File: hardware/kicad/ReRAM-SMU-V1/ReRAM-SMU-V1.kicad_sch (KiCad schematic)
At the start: 0 parts

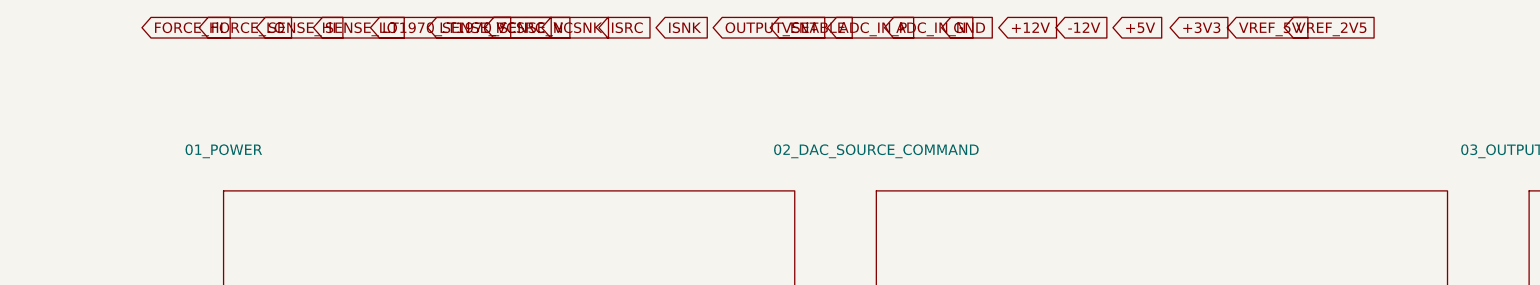
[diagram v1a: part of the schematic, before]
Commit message: Beta
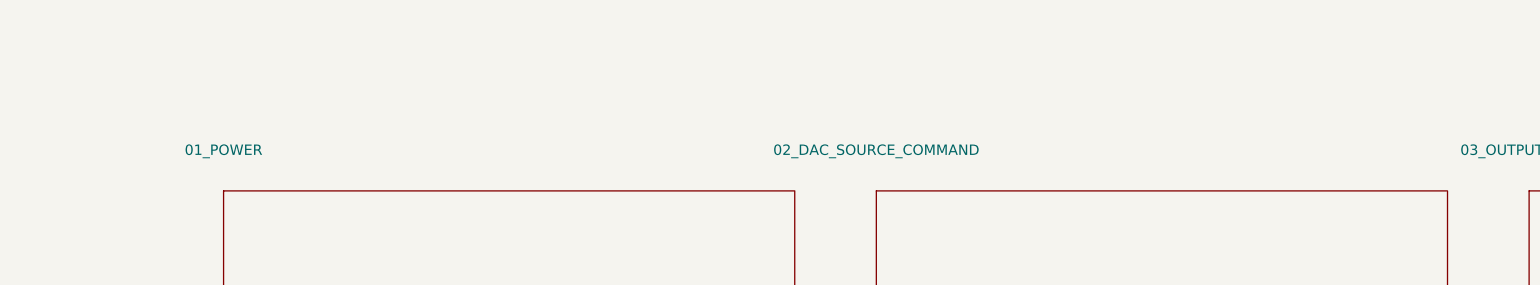
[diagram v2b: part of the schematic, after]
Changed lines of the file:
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@@
 		(property "Sheetfile" "sheets/09_DUT_CONNECTOR_GUARD.kicad_sch" (at 180 205 0) (effects (font (size 1.27 1.27))))
 	)
-	(global_label "FORCE_HI" (shape input) (at 10 10 0) (effects (font (size 1.27 1.27))) (property "Intersheetrefs" "${INTERSHEET_REFS}"))
-	(global_label "FORCE_LO" (shape input) (at 17 10 0) (effects (font (size 1.27 1.27))) (property "Intersheetrefs" "${INTERSHEET_REFS}"))
-	(global_label "SENSE_HI" (shape input) (at 24 10 0) (effects (font (size 1.27 1.27))) (property "Intersheetrefs" "${INTERSHEET_REFS}"))
-	(global_label "SENSE_LO" (shape input) (at 31 10 0) (effects (font (size 1.27 1.27))) (property "Intersheetrefs" "${INTERSHEET_REFS}"))
-	(global_label "LT1970_SENSE_P" (shape input) (at 38 10 0) (effects (font (size 1.27 1.27))) (property "Intersheetrefs" "${INTERSHEET_REFS}"))
-	(global_label "LT1970_SENSE_N" (shape input) (at 45 10 0) (effects (font (size 1.27 1.27))) (property "Intersheetrefs" "${INTERSHEET_REFS}"))
-	(global_label "VCSRC" (shape input) (at 52 10 0) (effects (font (size 1.27 1.27))) (property "Intersheetrefs" "${INTERSHEET_REFS}"))
-	(global_label "VCSNK" (shape input) (at 59 10 0) (effects (font (size 1.27 1.27))) (property "Intersheetrefs" "${INTERSHEET_REFS}"))
-	(global_label "ISRC" (shape input) (at 66 10 0) (effects (font (size 1.27 1.27))) (property "Intersheetrefs" "${INTERSHEET_REFS}"))
-	(global_label "ISNK" (shape input) (at 73 10 0) (effects (font (size 1.27 1.27))) (property "Intersheetrefs" "${INTERSHEET_REFS}"))
-	(global_label "OUTPUT_ENABLE" (shape input) (at 80 10 0) (effects (font (size 1.27 1.27))) (property "Intersheetrefs" "${INTERSHEET_REFS}"))
-	(global_label "VSET" (shape input) (at 87 10 0) (effects (font (size 1.27 1.27))) (property "Intersheetrefs" "${INTERSHEET_REFS}"))
-	(global_label "ADC_IN_P" (shape input) (at 94 10 0) (effects (font (size 1.27 1.27))) (property "Intersheetrefs" "${INTERSHEET_REFS}"))
-	(global_label "ADC_IN_N" (shape input) (at 101 10 0) (effects (font (size 1.27 1.27))) (property "Intersheetrefs" "${INTERSHEET_REFS}"))
-	(global_label "GND" (shape input) (at 108 10 0) (effects (font (size 1.27 1.27))) (property "Intersheetrefs" "${INTERSHEET_REFS}"))
-	(global_label "+12V" (shape input) (at 115 10 0) (effects (font (size 1.27 1.27))) (property "Intersheetrefs" "${INTERSHEET_REFS}"))
-	(global_label "-12V" (shape input) (at 122 10 0) (effects (font (size 1.27 1.27))) (property "Intersheetrefs" "${INTERSHEET_REFS}"))
-	(global_label "+5V" (shape input) (at 129 10 0) (effects (font (size 1.27 1.27))) (property "Intersheetrefs" "${INTERSHEET_REFS}"))
-	(global_label "+3V3" (shape input) (at 136 10 0) (effects (font (size 1.27 1.27))) (property "Intersheetrefs" "${INTERSHEET_REFS}"))
-	(global_label "VREF_5V" (shape input) (at 143 10 0) (effects (font (size 1.27 1.27))) (property "Intersheetrefs" "${INTERSHEET_REFS}"))
-	(global_label "VREF_2V5" (shape input) (at 150 10 0) (effects (font (size 1.27 1.27))) (property "Intersheetrefs" "${INTERSHEET_REFS}"))
 )
